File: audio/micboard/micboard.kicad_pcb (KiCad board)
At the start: 2 copper layers, 11 x 7.5 mm, 4 parts, among them P1 CONN_01X04, U1 MIC

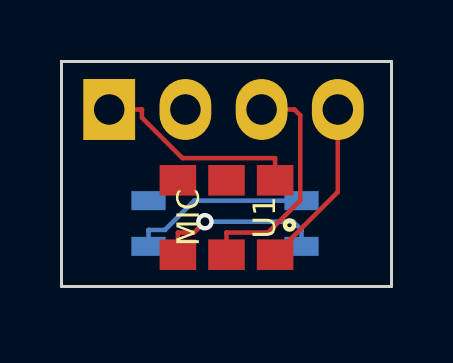
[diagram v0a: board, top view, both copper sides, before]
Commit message: finalizing audio board
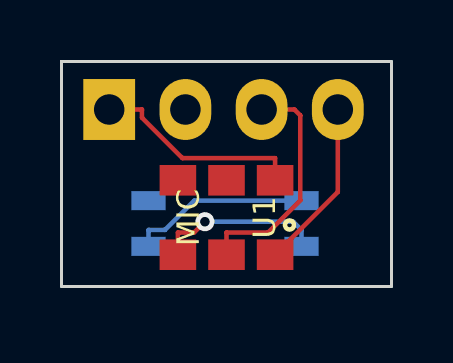
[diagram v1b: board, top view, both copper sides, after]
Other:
- board text added: "OUT GN - +"
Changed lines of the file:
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@@
-(kicad_pcb (version 4) (host pcbnew "(2014-09-08 BZR 5123)-product")
+(kicad_pcb (version 4) (host pcbnew "(2014-09-29 BZR 5155)-product")
   (general
     (links 7)
@@
     (area 148.007667 106.949999 160.792334 114.550001)
     (thickness 1.6)
-    (drawings 5)
+    (drawings 6)
     (tracks 24)
     (zones 0)
@@
       (net 3 +5V))
   )
+  (gr_text "OUT  GN  -   +" (at 154.813 110.49) (layer B.Mask)
+    (effects (font (size 0.75 0.75) (thickness 0.1875)) (justify mirror))
+  )
   (gr_line (start 149 114.5) (end 149 107) (angle 90) (layer Edge.Cuts) (width 0.1))
   (gr_line (start 160 114.5) (end 149 114.5) (angle 90) (layer Edge.Cuts) (width 0.1))
@@
   (gr_line (start 149 107) (end 160 107) (angle 90) (layer Edge.Cuts) (width 0.1))
   (gr_line (start 149 107) (end 149 107.1) (angle 90) (layer Edge.Cuts) (width 0.1))
-  (via (at 153.7802 112.3402) (size 0.5842) (layers F.Cu B.Cu) (net 1))
+  (via (at 153.7802 112.3402) (size 0.635) (layers F.Cu B.Cu) (net 1))
   (segment (start 153.4193 112.7011) (end 153.7802 112.3402) (width 0.1524) (layer F.Cu) (net 1))
   (segment (start 152.88 112.7011) (end 153.4193 112.7011) (width 0.1524) (layer F.Cu) (net 1))

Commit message: changed mic. board done...i hope
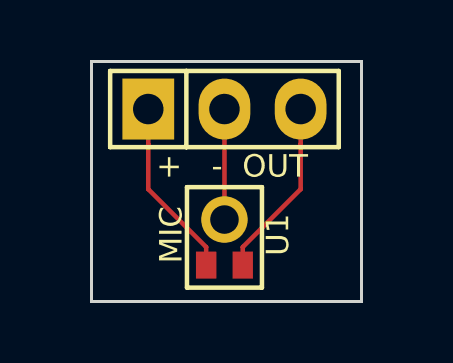
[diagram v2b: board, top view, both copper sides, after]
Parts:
- removed C1: 0.47uF, SMD_Packages:SMD-0603
- removed R1: 4K7, SMD_Packages:SMD-0603
- P1: value CONN_01X04 -> CONN_01X03; footprint Pin_Headers:Pin_Header_Straight_1x04 -> Pin_Headers:Pin_Header_Straight_1x03; moved to F.Cu
- moved U1 0.10 mm to (154.4, 112.3)
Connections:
- P1 pad 3: GAIN -> OUT
- U1 pad 2: GAIN -> GND
- U1 pad 3: Net-(C1-Pad1) -> +5V
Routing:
- net GAIN: track 7.84 -> 0.00 mm
- net Net-(C1-Pad2): track 6.05 -> 0.00 mm
- net Net-(C1-Pad1): track 5.67 -> 0.00 mm, vias 1 -> 0
- net GND: track 0.00 -> 3.68 mm
- net +5V: track 7.10 -> 6.00 mm
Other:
- board size 11 x 7.5 mm -> 9 x 8 mm
- board text added: "+ - OUT"
- board text removed: "OUT GN - +"
